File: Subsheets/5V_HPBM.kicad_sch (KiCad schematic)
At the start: 7 parts

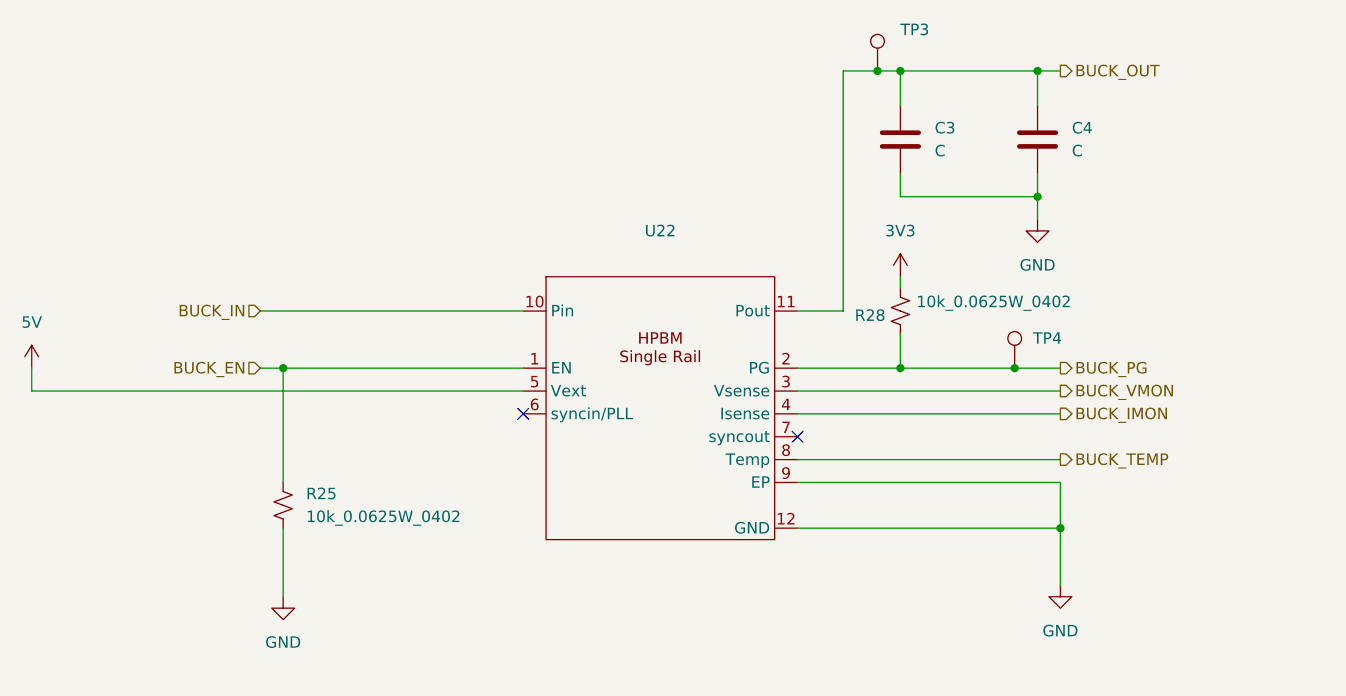
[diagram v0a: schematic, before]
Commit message: Schematic Update-1.1
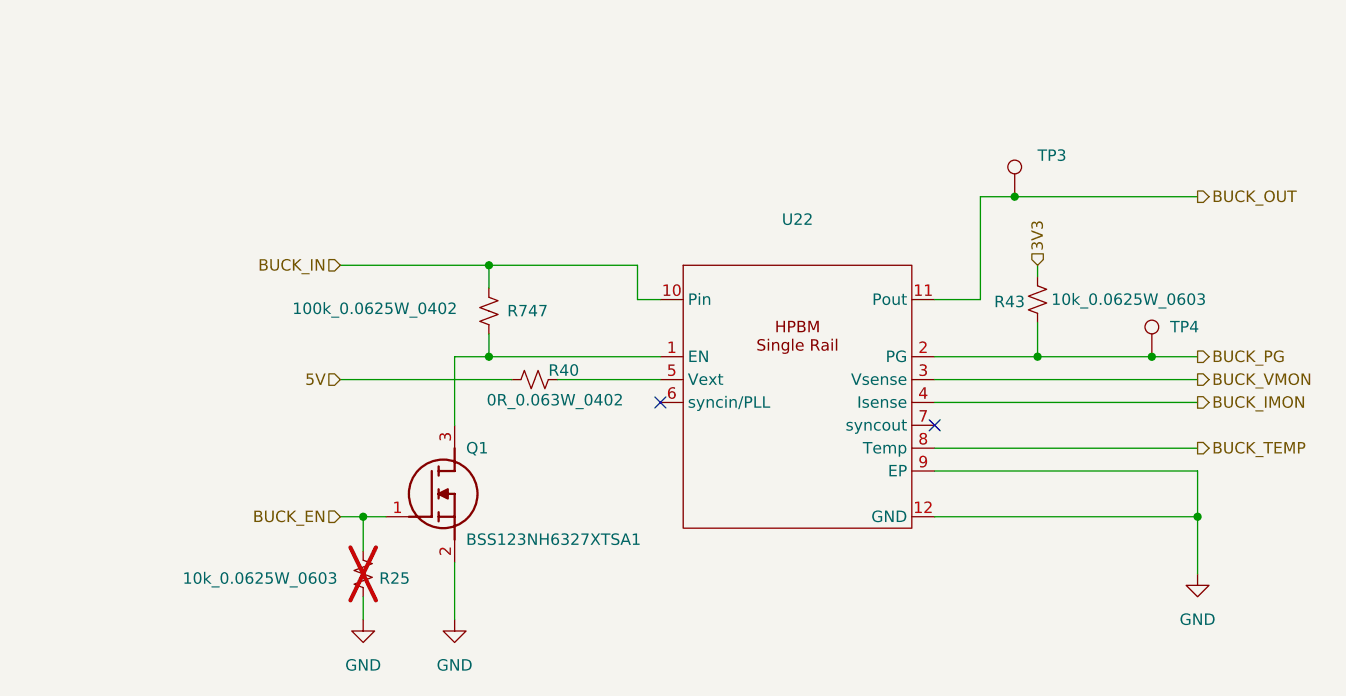
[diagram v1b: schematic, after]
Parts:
- removed C3, C4: C, symbol Device:C
- removed R28: 10k_0.0625W_0402, symbol Device:R_Small_US
- added Q1: BSS123NH6327XTSA1, SOT95P240X110-3N, symbol BSS123NH6327XTSA1:BSS123NH6327XTSA1
- added R40: 0R_0.063W_0402, Pixxel_Resistors:RES0402, symbol Device:R_Small_US
- added R43: 10k_0.0625W_0603, Pixxel_Resistors:RES0603, symbol Device:R_Small_US
- added R747: 100k_0.0625W_0402, Pixxel_Resistors:RES0402, symbol Device:R_Small_US
- R25: value 10k_0.0625W_0402 -> 10k_0.0625W_0603; footprint (none) -> Pixxel_Resistors:RES0603; Manufacturer Name (none) -> Vishay Dale; Manufacturer Part Number (none) -> TNPW060310K0BEEA; Price(INR) (none) -> 24.57; Temp_max (C) (none) -> 175; Temp_min (C) (none) -> -55; Vendor (none) -> Digikey; Vendor Part Number (none) -> TNP10.0KAATR-ND; now not fitted
- U22: value ~ -> (none)
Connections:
- net 3V3: now also R43.1
- net 5V: now also R40.2; no longer U22.5 (Vext)
- net BUCK_EN: now also Q1.1 (G); no longer U22.1 (EN)
- net BUCK_IN: now also R747.2
- net BUCK_PG: now also R43.2
- net GND: now also Q1.2 (S)
- new net: R40.1, U22.5 (Vext)
- new net: Q1.3 (D), R747.1, U22.1 (EN)
